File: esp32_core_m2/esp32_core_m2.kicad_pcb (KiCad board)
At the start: 4 copper layers, 30.3 x 22 mm, 37 parts, among them J1 NGFF_67P_M_KEY_Plug, U1 RT9013, U2 ESP32_C3_QFN_32, U3 ANT2051, U4 W25Q32JVSS, U5 IPEX_ANT, U6 WS2812_3535, Y1 Crystal_GND24

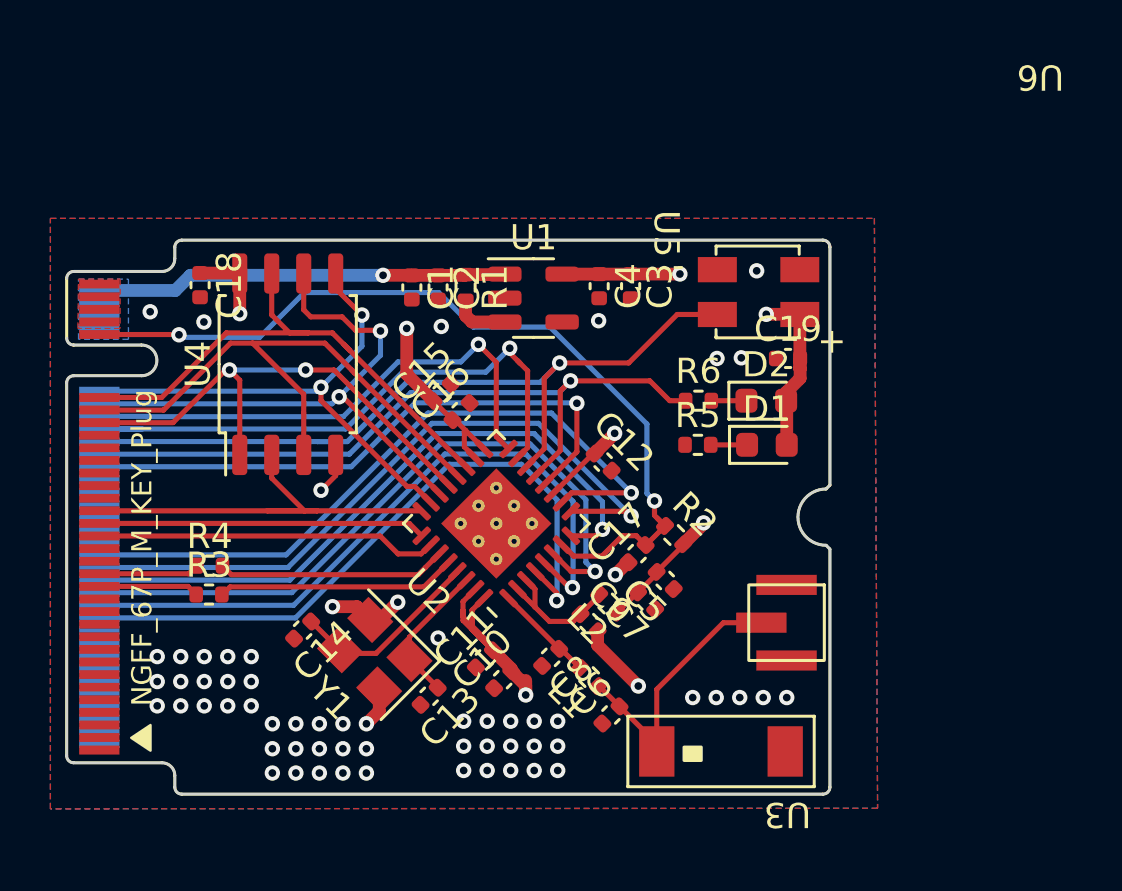
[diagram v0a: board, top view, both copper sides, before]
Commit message: update
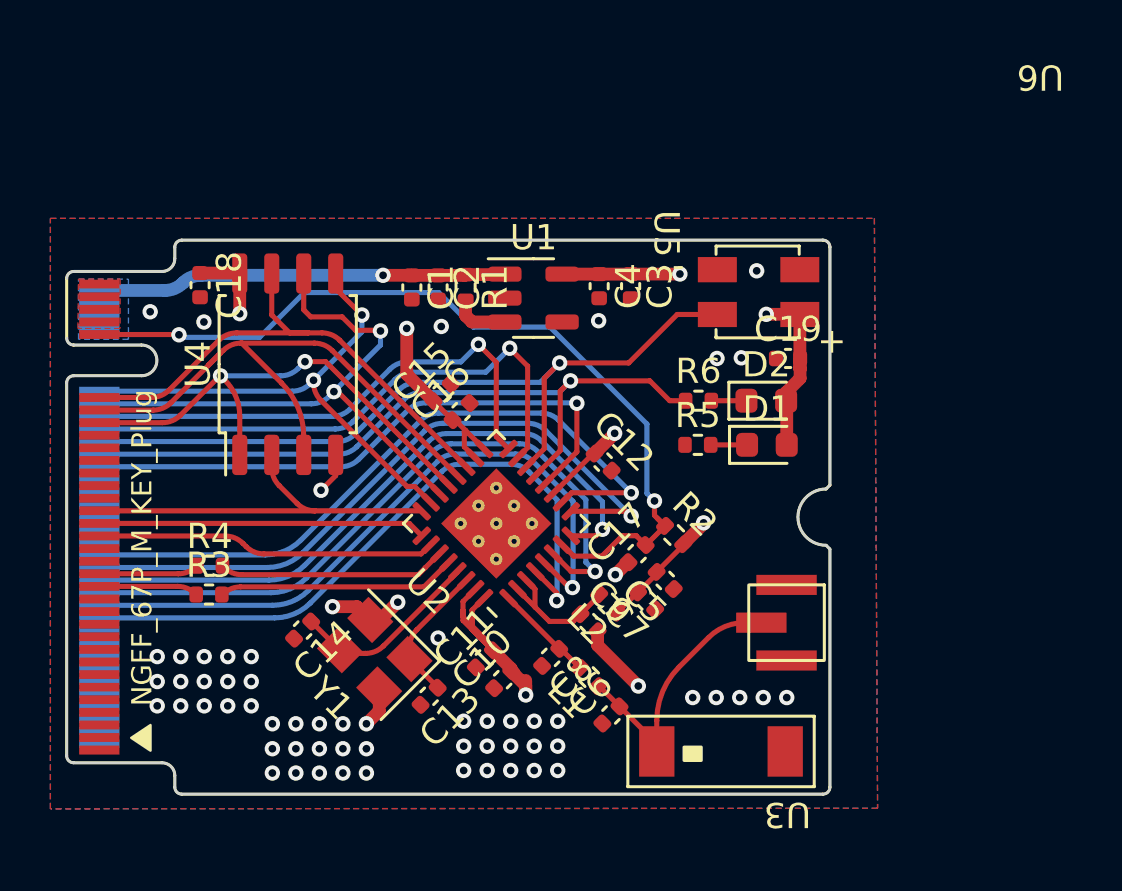
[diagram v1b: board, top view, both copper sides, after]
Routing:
- net +3V3: track 95.4 -> 93.3 mm
- net /GPIO9: track 24.3 -> 22.3 mm
- net /GPIO17: track 17.5 -> 15.9 mm
